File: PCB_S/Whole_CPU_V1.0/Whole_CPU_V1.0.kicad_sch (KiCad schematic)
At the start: 2188 parts, among them J1 Conn_01x21_Socket, J10 Conn_02x08_Odd_Even, J11 Conn_02x08_Odd_Even, J17 Conn_01x02_Pin, J18 Conn_01x02_Pin, J19 Conn_01x02_Pin, J2 Conn_01x21_Socket, J21 Conn_01x21_Socket, J22 Conn_01x21_Socket, J23 Conn_01x21_Socket, J24 Conn_01x21_Socket, J27 Conn_01x02_Pin, J28 Conn_01x02_Pin, J3 Conn_01x21_Socket, J4 Conn_01x21_Socket, J5 Conn_01x21_Socket, J6 Conn_01x21_Socket, J7 Conn_01x01_Pin, J8 Conn_01x01_Pin, J9 Conn_01x01_Pin, Q1 2N7002, Q10 2N7002, Q100 2N7002, Q1000 2N7002, Q1001 2N7002, Q1002 2N7002, Q1003 2N7002, Q1004 2N7002, Q1005 2N7002, Q1006 2N7002, Q1007 2N7002, Q1008 2N7002, Q1009 2N7002, Q101 2N7002, Q1010 2N7002, Q1011 2N7002, Q1012 2N7002, Q1013 2N7002, Q1014 2N7002, Q1015 2N7002, Q1016 2N7002, Q1017 2N7002, Q1018 2N7002, Q1019 2N7002, Q102 2N7002, Q1020 2N7002, Q1021 2N7002, Q1022 2N7002, Q1023 2N7002, Q1024 2N7002, Q1025 2N7002, Q1026 2N7002, Q1027 2N7002, Q1028 2N7002, Q1029 2N7002, Q103 2N7002, Q1030 2N7002, Q1031 2N7002, Q1032 2N7002, Q1033 2N7002, Q1034 2N7002, Q1035 2N7002, Q1036 2N7002, Q1037 2N7002, Q1038 2N7002, Q1039 2N7002, Q104 2N7002, Q1040 2N7002, Q1041 2N7002, Q1042 2N7002, Q1043 2N7002, Q1044 2N7002, Q1045 2N7002, Q1046 2N7002, Q1047 2N7002, Q1048 2N7002, Q1049 2N7002, Q105 2N7002, Q1050 2N7002, Q1051 2N7002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

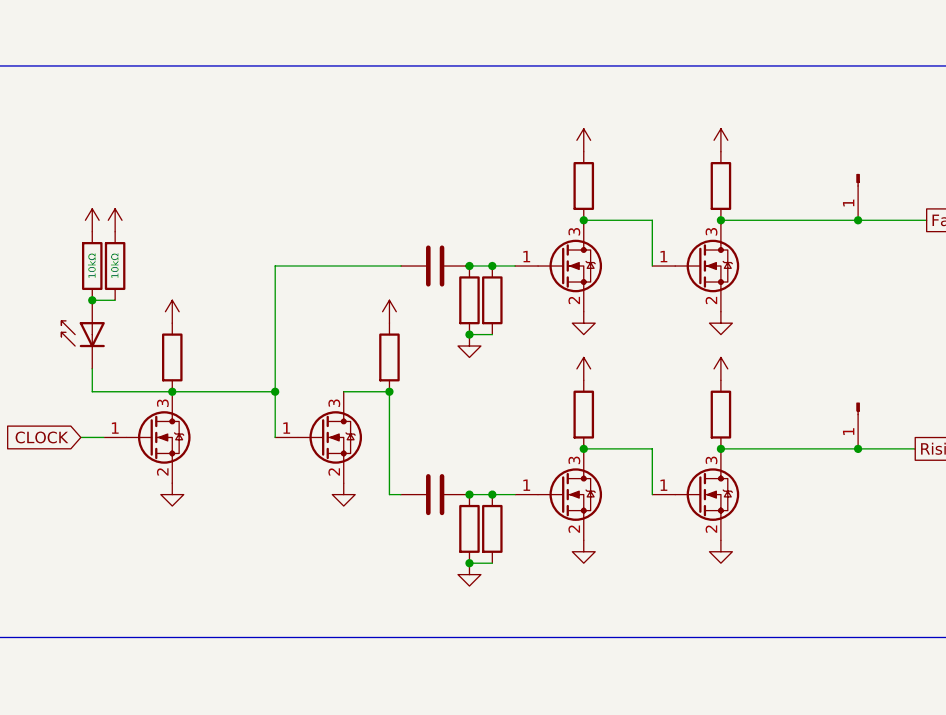
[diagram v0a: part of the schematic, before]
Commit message: order tomorrow
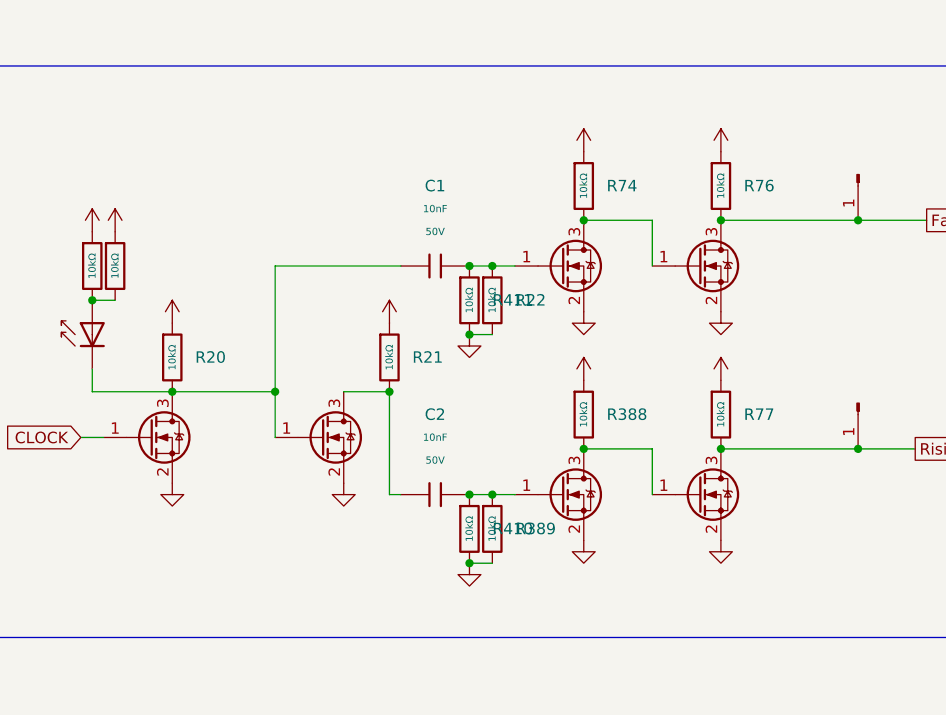
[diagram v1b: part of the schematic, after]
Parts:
- removed C1, C2: C, Capacitor_THT:C_Disc_D4.7mm_W2.5mm_P5.00mm, symbol Device:C
- removed R20, R21, R22, R388, R389, R410, R411, R74, R76, R77: R, Resistor_THT:R_Axial_DIN0207_L6.3mm_D2.5mm_P7.62mm_Horizontal, symbol Device:R
- added C1, C2: 10nF, PCM_JLCPCB:C_1206, symbol PCM_JLCPCB-Capacitors:1206,10nF
- added R20, R21, R22, R388, R389, R410, R411, R74, R76, R77: 10kΩ, PCM_JLCPCB:R_1206, symbol PCM_JLCPCB-Resistors:1206,10kΩ
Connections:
- net Faling Edge: now also R76.2
- net GND: now also R22.2, R389.2, R410.2, R411.2
- net Rising Edge: now also R77.2
- net VCC: now also R20.1, R21.1, R388.1, R74.1, R76.1, R77.1
- net at Q607.1 (G): now also C2.2, R389.1, R410.1
- net at Q606.3 (D), Q609.1 (G): now also R74.2
- net at Q607.3 (D), Q608.1 (G): now also R388.2
- net at D40.1, Q604.3 (D), Q605.1 (G): now also C1.1, R20.2
- net at Q606.1 (G): now also C1.2, R22.1, R411.1
- net at Q605.3 (D): now also C2.1, R21.2
